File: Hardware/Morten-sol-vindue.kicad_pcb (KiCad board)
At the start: 2 copper layers, 40 parts, among them J1 Conn_01x04, J2 CUI_PJ-079BH, J3 SJ-43514-SMT, J4 AudioJack4, U1 LV2862YDDCR, U2 AMS1117-3.3, U3 ATtiny412-SS, U4 LM358, U5 SHT4x

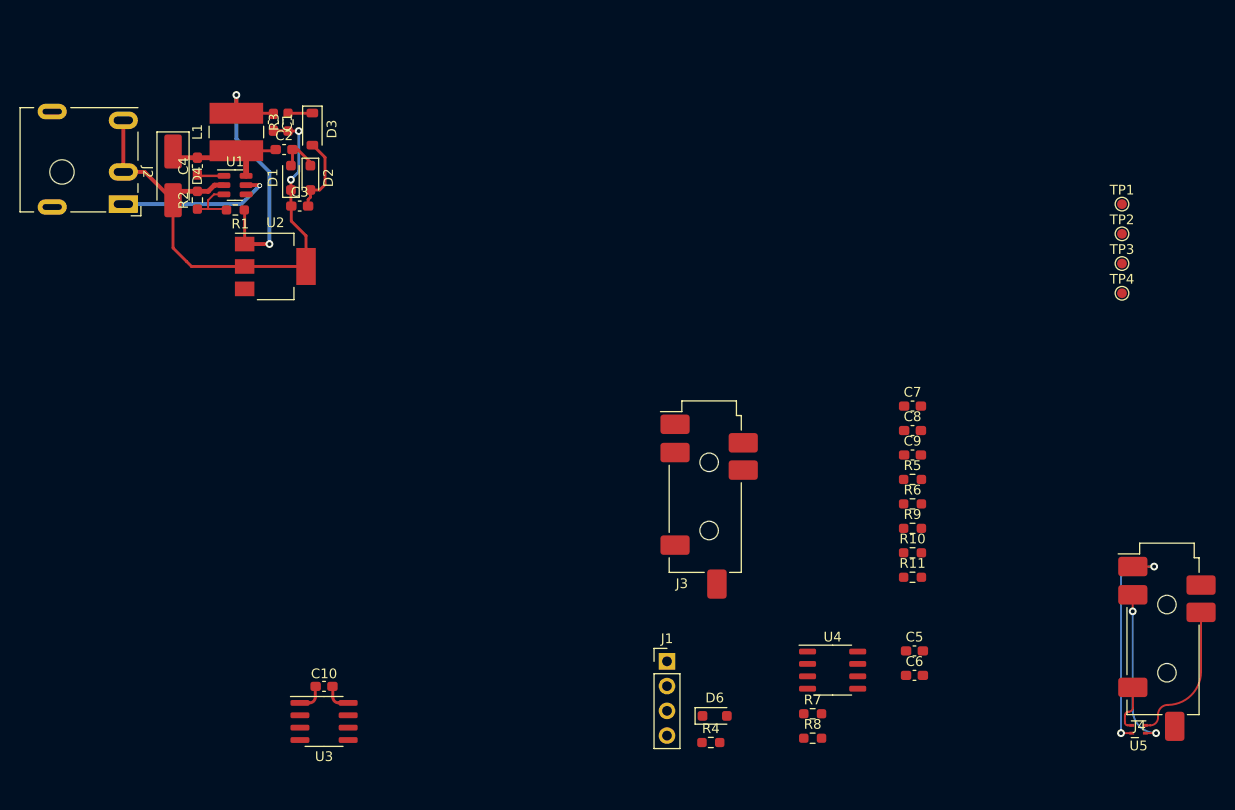
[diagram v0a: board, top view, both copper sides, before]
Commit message: Initial layout
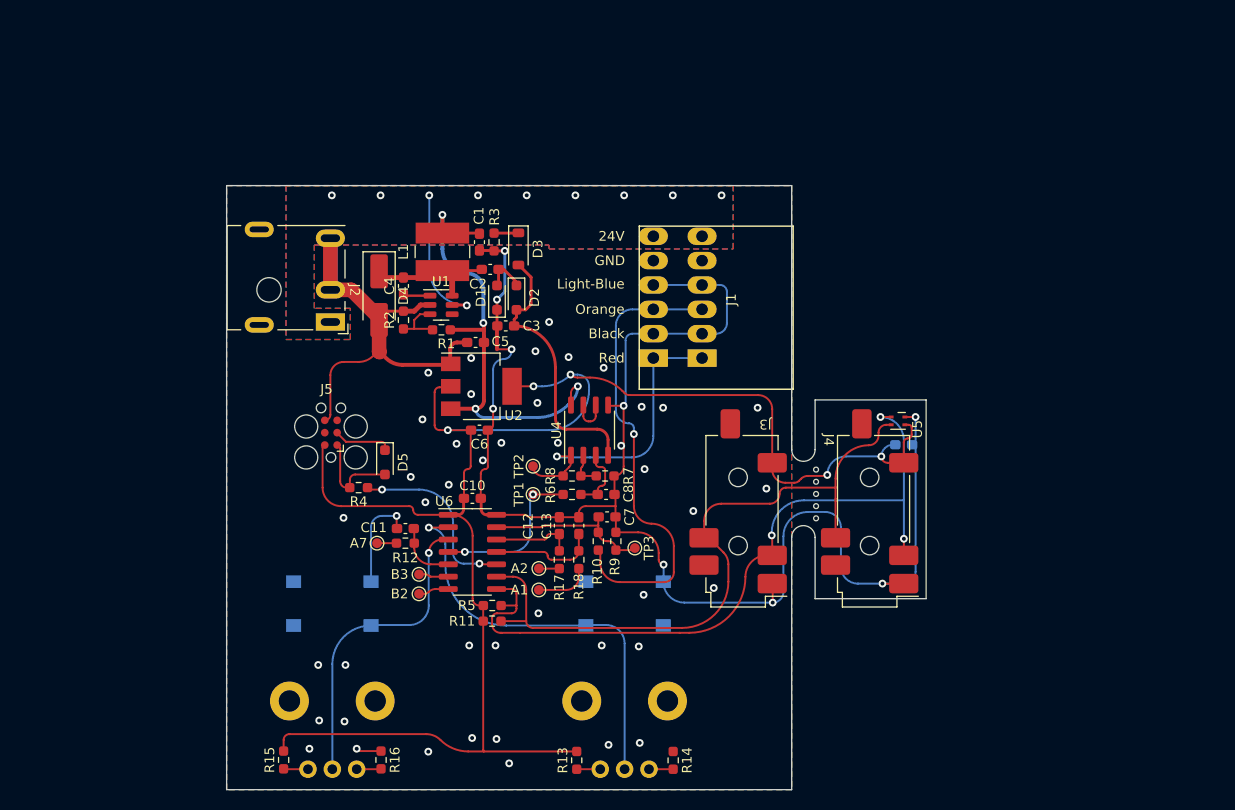
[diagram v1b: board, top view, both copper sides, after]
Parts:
- removed D6: BAT54WS, Diode_SMD:D_SOD-323_HandSoldering
- removed TP4: PA7, TestPoint:TestPoint_Pad_D1.0mm
- removed U3: ATtiny412-SS, Package_SO:SOIC-8_3.9x4.9mm_P1.27mm
- added A1: PA7, TestPoint:TestPoint_Pad_D1.0mm, F.Cu at (171.1, 91.5)
- added A2: PA7, TestPoint:TestPoint_Pad_D1.0mm, F.Cu at (171.1, 89.3)
- added A7: PA7, TestPoint:TestPoint_Pad_D1.0mm, F.Cu at (154.4, 86.7)
- added B2: PA7, TestPoint:TestPoint_Pad_D1.0mm, F.Cu at (158.8, 91.9)
- added B3: PA7, TestPoint:TestPoint_Pad_D1.0mm, F.Cu at (158.8, 89.9)
- added C11: 100nF, Capacitor_SMD:C_0603_1608Metric_Pad1.08x0.95mm_HandSolder, F.Cu at (157.3, 85.2)
- added C12: 100nF, Capacitor_SMD:C_0603_1608Metric_Pad1.08x0.95mm_HandSolder, F.Cu at (173.2, 84.9)
- added C13: 100nF, Capacitor_SMD:C_0603_1608Metric_Pad1.08x0.95mm_HandSolder, F.Cu at (175.2, 84.9)
- added D5: BAT54WS, Diode_SMD:D_SOD-323_HandSoldering, F.Cu at (155.2, 78.4)
- added G***: LOGO, graphics:kiwi, F.Cu at (147.2, 92.5)
- added G***: LOGO, graphics:kiwi, B.Cu at (145.6, 85.0)
- added J5: AVR-UPDI-6, Connector:Tag-Connect_TC2030-IDC-FP_2x03_P1.27mm_Vertical, F.Cu at (149.7, 75.4)
- added R12: 100R, Resistor_SMD:R_0603_1608Metric_Pad0.98x0.95mm_HandSolder, F.Cu at (157.3, 86.7)
- added R13: 33k, Resistor_SMD:R_0603_1608Metric_Pad0.98x0.95mm_HandSolder, F.Cu at (174.9, 109.0)
- added R14: 1k, Resistor_SMD:R_0603_1608Metric_Pad0.98x0.95mm_HandSolder, F.Cu at (184.8, 109.0)
- added R15: 33k, Resistor_SMD:R_0603_1608Metric_Pad0.98x0.95mm_HandSolder, F.Cu at (144.8, 109.0)
- added R16: 1k, Resistor_SMD:R_0603_1608Metric_Pad0.98x0.95mm_HandSolder, F.Cu at (154.8, 109.0)
- added R17: 100R, Resistor_SMD:R_0603_1608Metric_Pad0.98x0.95mm_HandSolder, F.Cu at (173.2, 88.4)
- added R18: 100R, Resistor_SMD:R_0603_1608Metric_Pad0.98x0.95mm_HandSolder, F.Cu at (175.2, 88.4)
- added REF**: Pin_D1.0mm_L10.0mm, Connector_Pin:Pin_D1.0mm_L10.0mm, F.Cu at (199.5, 79.2)
- added REF**1: Pin_D1.0mm_L10.0mm, Connector_Pin:Pin_D1.0mm_L10.0mm, F.Cu at (199.5, 80.4)
- added REF**2: Pin_D1.0mm_L10.0mm, Connector_Pin:Pin_D1.0mm_L10.0mm, F.Cu at (199.5, 81.7)
- added REF**3: Pin_D1.0mm_L10.0mm, Connector_Pin:Pin_D1.0mm_L10.0mm, F.Cu at (199.5, 82.9)
- added REF**4: Pin_D1.0mm_L10.0mm, Connector_Pin:Pin_D1.0mm_L10.0mm, F.Cu at (199.5, 84.2)
- added RV1: 100K, Potentiometer_THT:Potentiometer_Bourns_PTV09A-1_Single_Vertical, B.Cu at (177.3, 109.9)
- added RV2: 100K, Potentiometer_THT:Potentiometer_Bourns_PTV09A-1_Single_Vertical, B.Cu at (147.3, 109.9)
- added SW1: SW_Push, Button_Switch_SMD:SW_Push_1P1T_NO_6x6mm_H9.5mm, B.Cu at (179.8, 92.9)
- added SW2: SW_Push, Button_Switch_SMD:SW_Push_1P1T_NO_6x6mm_H9.5mm, B.Cu at (149.8, 92.9)
- added U6: ATtiny414-SS, Package_SO:SOIC-14_3.9x8.7mm_P1.27mm, F.Cu at (164.2, 87.6)
- C9: moved to B.Cu
- J1: value Conn_01x04 -> CUI TBL009-254-06xx; footprint Connector_PinHeader_2.54mm:PinHeader_1x04_P2.54mm_Vertical -> TerminalBlock_Phoenix:TerminalBlock_Phoenix_PTSM-0,5-6-2.5-H-THR_1x06_P2.50mm_Horizontal
- R6: value 100R -> 1k
- R7: value 100k -> 33k
- R8: value 33k -> 100k
- moved TP1 67.4 mm to (170.4, 81.7), turned to 90 degrees
- moved TP2 65.0 mm to (170.4, 78.8), turned to 90 degrees
- moved TP3 57.9 mm to (180.9, 87.2), turned to -90 degrees
- moved C5 55.1 mm to (164.6, 66.1)
- moved C6 51.3 mm to (164.9, 75.1), turned to 180 degrees
- moved R5 45.0 mm to (166.3, 93.1)
- moved R4 44.6 mm to (152.6, 81.0), turned to 180 degrees
- moved R11 43.4 mm to (166.2, 94.7)
- moved U5 40.1 mm to (207.9, 74.2), turned to 0 degrees
- moved R8 36.5 mm to (174.4, 79.8), turned to 180 degrees
- moved U4 35.1 mm to (176.2, 75.1), turned to 90 degrees
- moved R6 35.0 mm to (174.4, 81.7)
- moved J4 34.1 mm to (205.0, 82.4), turned to 180 degrees
- moved C7 33.3 mm to (178.1, 84.0), turned to 180 degrees
- moved R7 32.4 mm to (177.8, 79.8)
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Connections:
- net /Analog/Ain renamed Net-(U4A-+)
- net /MCU/A3 renamed Net-(U6-PA3)
- net /MCU/Aout renamed Net-(U6-PA6)
- net /SCL renamed SCL
- net /SDA renamed SDA
- J1 pad 1: +3V3 -> /0-10V out
- J1 pad 2: /MCU/Adapter TX -> GND
- J1 pad 3: /MCU/Adapter RX -> /0-10V in
- R4 pad 1: /MCU/UPDI -> /UPDI
- R4 pad 2: /MCU/Adapter RX -> /Adapter RX
- R7 pad 2: /0-10V out -> GND
- R8 pad 2: /Analog/0V -> /0-10V out
- U4 pad 5: /Analog/0V -> GND
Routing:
- net +3V3: track 7.90 -> 174.1 mm, vias 0 -> 5
- net GND: track 80.3 -> 228.5 mm, vias 4 -> 53
- net SDA: track 16.6 -> 76.8 mm, vias 2 -> 3
- net SCL: track 14.9 -> 70.8 mm
- net /0-10V in: track 0.00 -> 48.7 mm, vias 0 -> 1
- net closed_SP: track 0.00 -> 42.4 mm, vias 0 -> 1
- net open_SP: track 0.00 -> 32.0 mm, vias 0 -> 1
- net /0-10V out: track 0.00 -> 31.6 mm, vias 0 -> 1
- net -12VA: track 8.09 -> 28.0 mm
- net /UPDI: track 0.00 -> 18.8 mm, vias 0 -> 2
- net +12VA: track 30.6 -> 49.1 mm, vias 2 -> 4
- net Net-(U6-PA3): track 0.00 -> 16.9 mm
- net Net-(U6-PA6): track 0.00 -> 16.7 mm, vias 0 -> 2
- net Net-(U6-PA1): track 0.00 -> 11.1 mm
- net /Adapter RX: track 0.00 -> 9.87 mm
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- added copper zone on B.Cu, net +24V
- added copper zone on F.Cu, net +24V
- added copper zone on B.Cu, net GND
- added copper zone on F.Cu, net GND
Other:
- board outline added: 71.8 x 62 mm
- board text added: "24V"
- board text added: "Black"
- board text added: "GND"
- board text added: "Light-Blue"
- board text added: "Orange"
- board text added: "Red"

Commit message: Re-layout
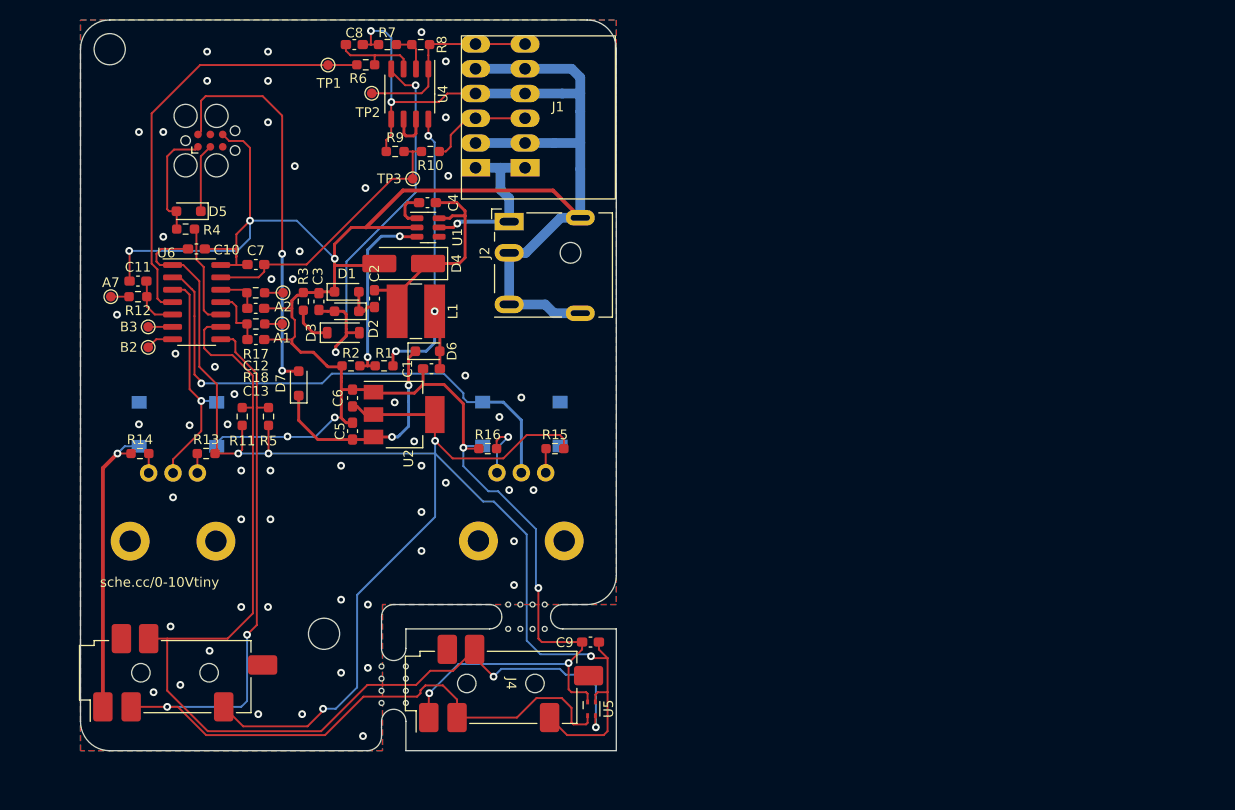
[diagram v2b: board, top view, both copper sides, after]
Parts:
- removed the G*** at (147.2, 92.5)
- removed the G*** at (145.6, 85.0)
- removed the REF** at (199.5, 79.2)
- removed REF**1, REF**2, REF**3, REF**4: Pin_D1.0mm_L10.0mm, Connector_Pin:Pin_D1.0mm_L10.0mm
- added D6: BAT54WS, Diode_SMD:D_SOD-323_HandSoldering, F.Cu at (159.6, 67.0)
- added D7: BAT54WS, Diode_SMD:D_SOD-323_HandSoldering, F.Cu at (146.4, 70.3)
- added G***: LOGO, graphics:kiwi, F.Cu at (150.2, 85.0)
- added G***: LOGO, graphics:kiwi, B.Cu at (150.2, 85.0)
- added REF**: 2.5mm_slot, mouse_bites:2.5mm_slot, F.Cu at (173.5, 95.5)
- added REF**: MountingHole_3.2mm_M3_DIN965, MountingHole:MountingHole_3.2mm_M3_DIN965, F.Cu at (127.0, 36.0)
- added REF**: MountingHole_3.2mm_M3_DIN965, MountingHole:MountingHole_3.2mm_M3_DIN965, F.Cu at (149.0, 96.0)
- added REF**: 2.5mm_slot, mouse_bites:2.5mm_slot, F.Cu at (157.4, 97.5)
- C9: moved to F.Cu
- moved R14 63.1 mm to (130.1, 77.5), turned to 0 degrees
- moved J3 59.4 mm to (134.8, 100.0), turned to 90 degrees
- moved C8 52.9 mm to (152.1, 35.5)
- moved RV1 51.3 mm to (136.0, 79.5), turned to -90 degrees
- moved R7 49.6 mm to (155.5, 35.5), turned to 180 degrees
- moved SW1 49.4 mm to (134.0, 74.5), turned to 180 degrees
- moved R13 49.4 mm to (136.9, 77.5), turned to 0 degrees
- moved R6 48.9 mm to (153.3, 37.6)
- moved TP1 48.8 mm to (149.4, 37.6), turned to -90 degrees
- moved R8 46.9 mm to (158.9, 35.5), turned to 0 degrees
- moved R9 46.0 mm to (156.3, 46.5), turned to 0 degrees
- moved C7 44.4 mm to (142.0, 58.1), turned to 0 degrees
- moved TP3 44.2 mm to (158.1, 49.3), turned to 0 degrees
- moved R10 43.6 mm to (159.9, 46.5), turned to 180 degrees
- moved U5 43.2 mm to (176.4, 103.7), turned to 90 degrees
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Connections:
- C5 pad 2: +12VA -> Net-(D6-K)
- J1 pad 1: /0-10V out -> +24V
- J1 pad 6: +24V -> /0-10V out
- J5 pad 2: +3V3 -> VBUS
- U2 pad 3: +12VA -> Net-(D6-K)
- U6 pad 2: closed_SP -> open_SP
- U6 pad 3: open_SP -> closed_SP
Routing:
- net GND: track 228.5 -> 339.7 mm, vias 53 -> 68
- net VBUS: track 0.00 -> 40.8 mm, vias 0 -> 2
- net SCL: track 70.8 -> 109.9 mm, vias 0 -> 2
- net /0-10V in: track 48.7 -> 10.9 mm, vias 1 -> 0
- net SDA: track 76.8 -> 105.9 mm, vias 3 -> 2
- net Net-(U6-PA6): track 16.7 -> 44.1 mm, vias 2 -> 0
- net Net-(D6-K): track 0.00 -> 23.2 mm, vias 0 -> 2
- net open_SP: track 32.0 -> 53.5 mm
- net closed_SP: track 42.4 -> 23.6 mm
- net -12VA: track 28.0 -> 42.8 mm, vias 0 -> 2
- net Net-(U1-FB): track 5.81 -> 19.3 mm, vias 0 -> 2
- net +12VA: track 49.1 -> 35.8 mm, vias 4 -> 3
- net Net-(U6-PA3): track 16.9 -> 28.9 mm
- net /0-10V out: track 31.6 -> 20.3 mm, vias 1 -> 0
- net Net-(D4-K): track 12.6 -> 23.7 mm
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- removed copper zone on B.Cu, net +24V
- removed copper zone on F.Cu, net +24V
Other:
- board size 71.8 x 62 mm -> 55 x 75 mm
- board text added: "sche.cc/0-10Vtiny"
- board text removed: "24V"
- board text removed: "Black"
- board text removed: "GND"
- board text removed: "Light-Blue"
- board text removed: "Orange"
- board text removed: "Red"
